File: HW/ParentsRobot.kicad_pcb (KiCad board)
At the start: 2 copper layers, 26 parts, among them J1 Front_LEDs, J2 POWER_INPUT, J3 UART_BOOT, J4 LEFT_MOTORS, J5 RIGHT_MOTORS, Q1 BS170, SW1 RESET, SW2 BOOT, SW3 ChannelSelection, U1 AMS1117-3.3, U2 ESP32-WROOM-32, U3 L293D

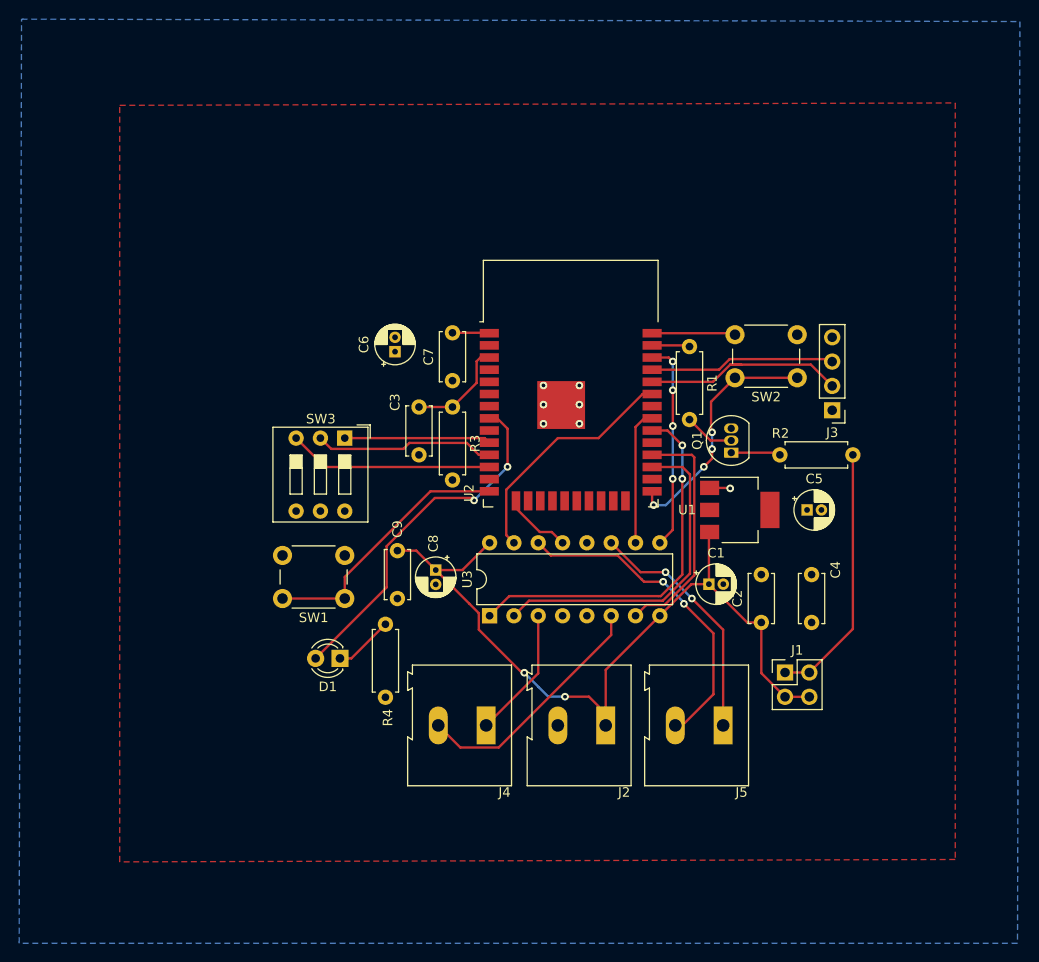
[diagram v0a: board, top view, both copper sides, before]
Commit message: Hardware done
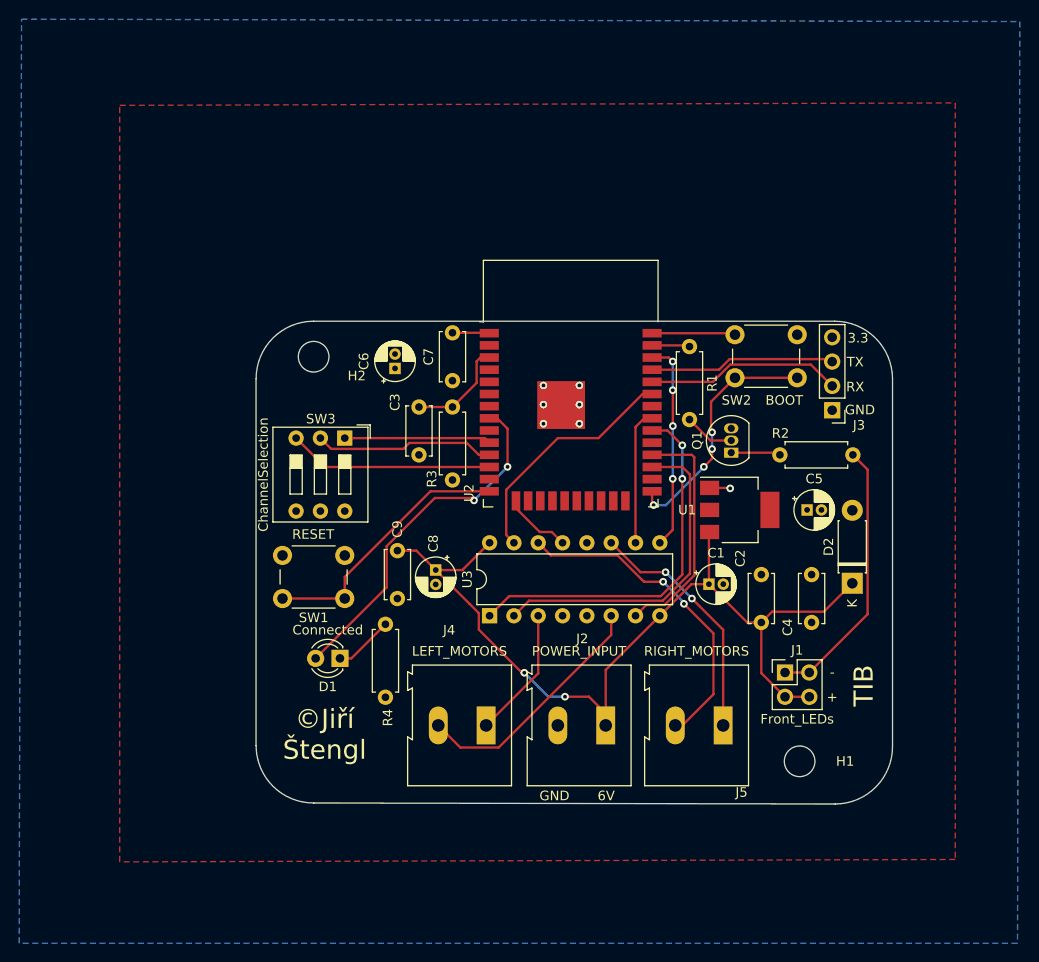
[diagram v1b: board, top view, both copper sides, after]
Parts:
- added D2: D, Diode_THT:D_DO-41_SOD81_P7.62mm_Horizontal, F.Cu at (169.5, 68.4)
- added H1: MountingHole, MountingHole:MountingHole_3.2mm_M3, F.Cu at (164.0, 87.0)
- added H2: MountingHole, MountingHole:MountingHole_3.2mm_M3, F.Cu at (113.2, 44.8)
- moved C4 5.00 mm to (165.2, 67.5), turned to -90 degrees
- moved C6 1.75 mm to (121.8, 46.0)
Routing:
- net VCC: track 82.1 -> 93.3 mm
- net Net-(R2-Pad2): track 27.1 -> 28.4 mm
- net Net-(J3-Pad2): track 21.6 -> 20.5 mm
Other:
- board outline added: 66.5 x 50.4 mm
- board text added: "+"
- board text added: "-"
- board text added: "3.3"
- board text added: "6V"
- board text added: "GND"
- board text added: "RX"
- board text added: "TIB"
- board text added: "TX"
- board text added: "©Jiří Štengl"
